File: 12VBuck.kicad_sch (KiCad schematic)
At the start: 10 parts, among them U1 LMR51635XDDCR

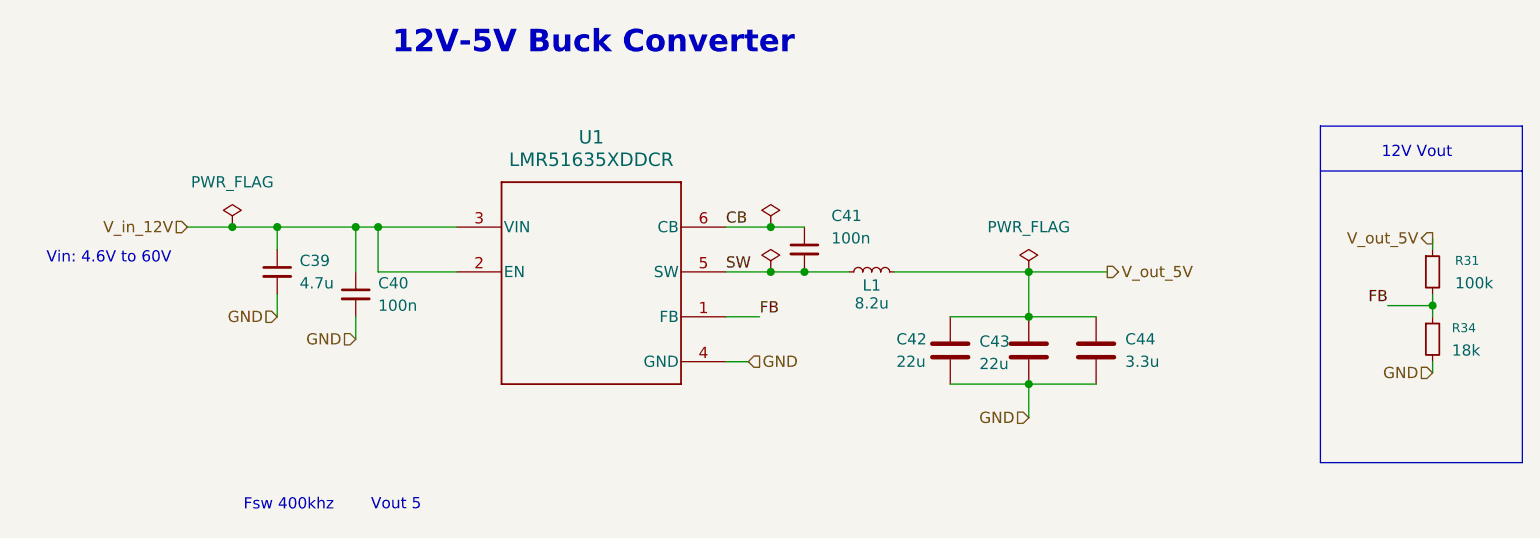
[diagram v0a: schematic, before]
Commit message: shoupu review done
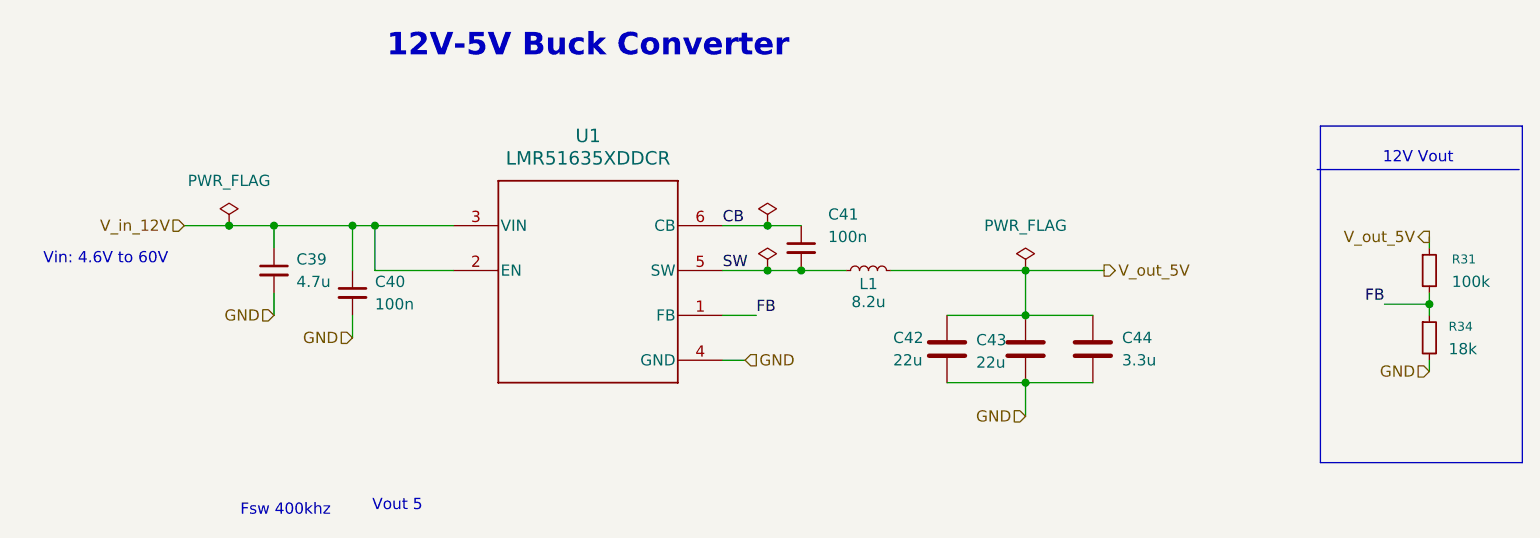
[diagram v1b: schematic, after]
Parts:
- U1: footprint DDC0006A-MFG -> (none)

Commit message: review council
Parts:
- C41: footprint Capacitor_SMD:C_0603_1608Metric -> Capacitor_SMD:C_0603_1608Metric_Pad1.08x0.95mm_HandSolder
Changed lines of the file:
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@@
 			)
 		)
-		(property "Footprint" "Capacitor_SMD:C_0603_1608Metric"
+		(property "Footprint" "Capacitor_SMD:C_0603_1608Metric_Pad1.08x0.95mm_HandSolder"
 			(at 158.75 86.36 0)
 			(hide yes)

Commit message: meh
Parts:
- C42, C43: footprint Capacitor_SMD:C_1210_3225Metric_Pad1.33x2.70mm_HandSolder -> Capacitor_SMD:C_1206_3216Metric_Pad1.33x1.80mm_HandSolder
- U1: footprint (none) -> LHRS_ICs:DDC0006A-MFG
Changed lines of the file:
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@@
 			)
 		)
-		(property "Footprint" "Capacitor_SMD:C_1210_3225Metric_Pad1.33x2.70mm_HandSolder"
+		(property "Footprint" "Capacitor_SMD:C_1206_3216Metric_Pad1.33x1.80mm_HandSolder"
 			(at 176.2252 101.6 0)
 			(hide yes)
@@
 			)
 		)
-		(property "Footprint" "Capacitor_SMD:C_1210_3225Metric_Pad1.33x2.70mm_HandSolder"
+		(property "Footprint" "Capacitor_SMD:C_1206_3216Metric_Pad1.33x1.80mm_HandSolder"
 			(at 185.1152 101.6 0)
 			(hide yes)
@@
 			)
 		)
-		(property "Footprint" ""
+		(property "Footprint" "LHRS_ICs:DDC0006A-MFG"
 			(at 119.38 83.82 0)
 			(hide yes)

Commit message: usbc,ldo,buck
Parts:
- L1: footprint LHRS_Power:XAL5050822MEC -> LHRS_Passives:74439369082
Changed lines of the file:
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@@
 			)
 		)
-		(property "Footprint" "LHRS_Power:XAL5050822MEC"
+		(property "Footprint" "LHRS_Passives:74439369082"
 			(at 166.37 88.9 0)
 			(hide yes)
